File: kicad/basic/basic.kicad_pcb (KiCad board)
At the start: 2 copper layers, 50 x 50 mm, 20 parts, among them P2 CONN_01X15, P3 CONN_01X15, P4 CONN_01X06, P5 CONN_01X01, P6 CONN_01X01, P7 CONN_01X01, P8 CONN_01X01, P9 CONN_01X06, SW1 SW_PUSH, SW2 SW_PUSH

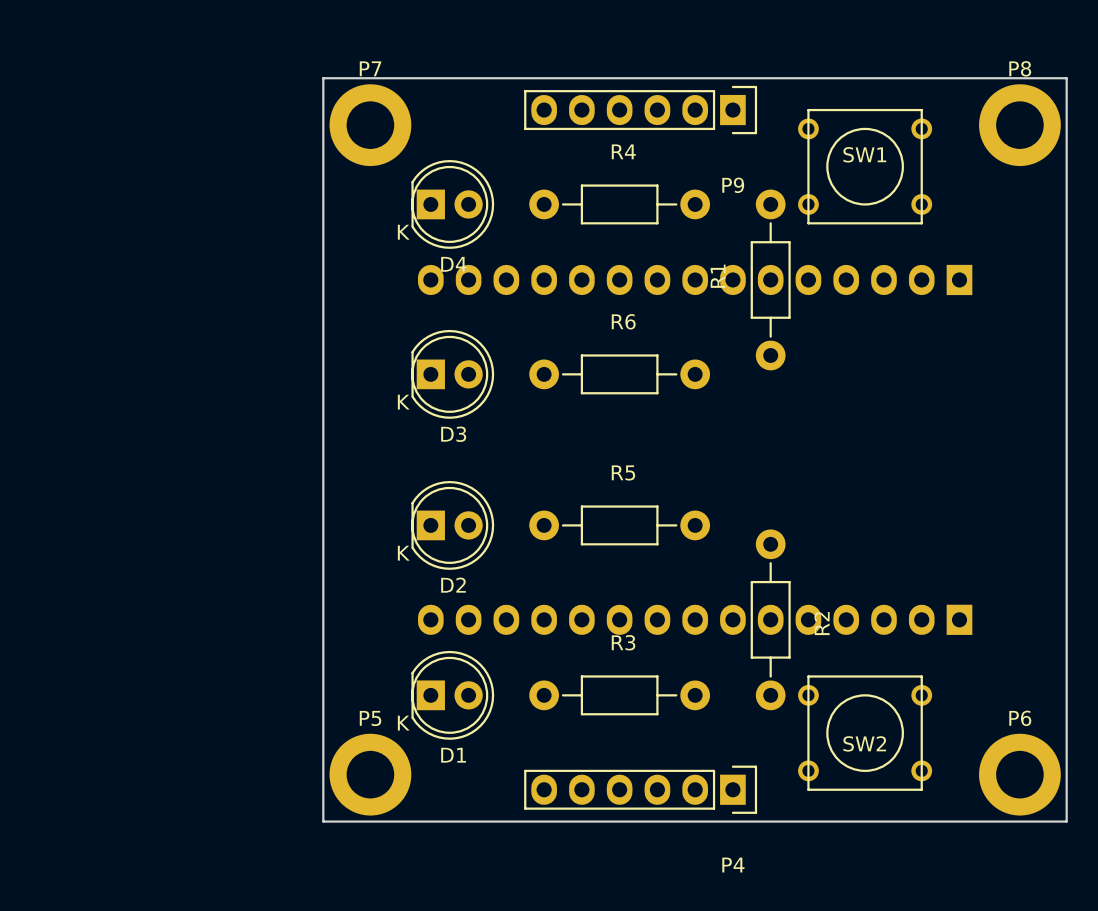
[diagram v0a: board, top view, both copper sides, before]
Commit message: Labeling
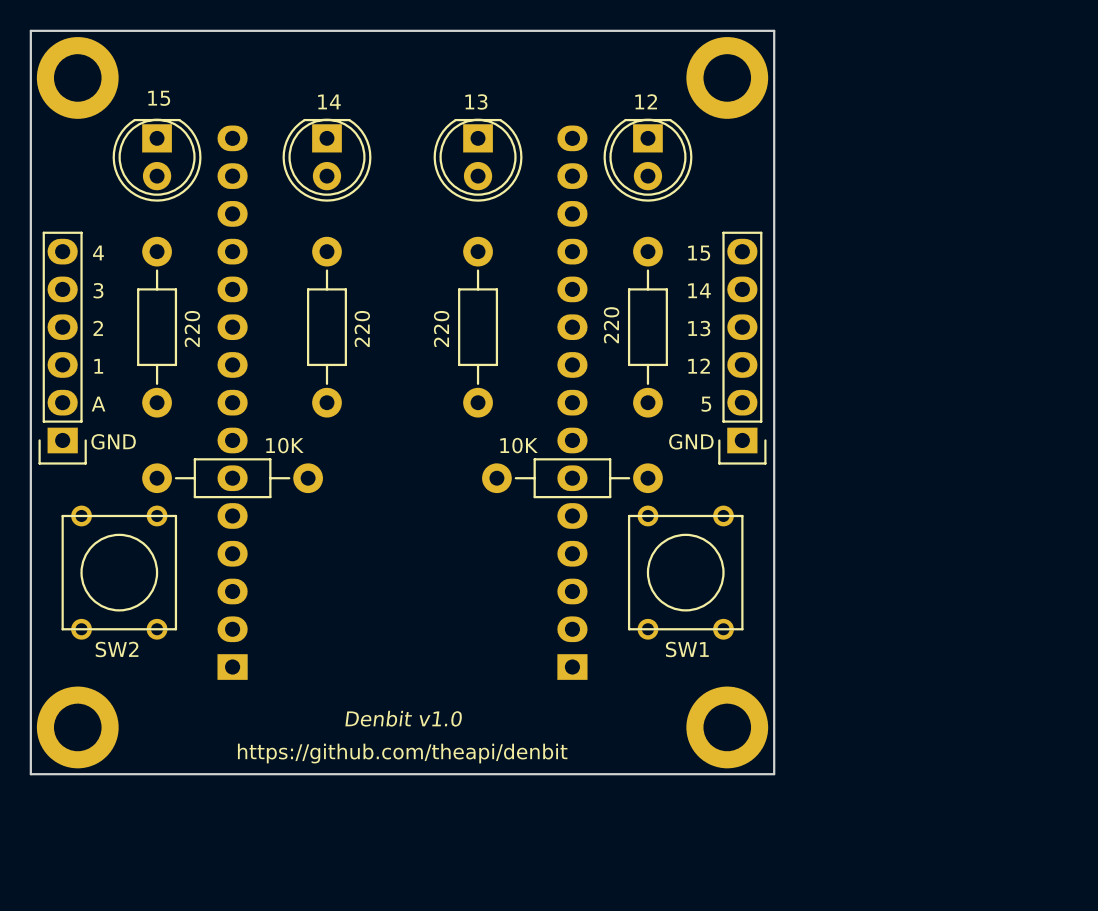
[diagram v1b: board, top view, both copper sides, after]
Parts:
- moved P6 63.5 mm to (123.5, 118.7), turned to 270 degrees
- moved SW2 51.3 mm to (126.3, 108.3), turned to 90 degrees
- moved P4 50.8 mm to (122.5, 99.4), turned to 90 degrees
- moved P5 50.8 mm to (123.5, 75.0), turned to 270 degrees
- moved P2 49.0 mm to (133.9, 114.6), turned to 90 degrees
- moved P8 45.0 mm to (167.2, 118.7), turned to 270 degrees
- moved D1 41.7 mm to (128.8, 79.0), turned to 270 degrees
- moved R3 39.6 mm to (128.8, 86.7), turned to 270 degrees
- moved P3 36.8 mm to (156.8, 114.6), turned to 90 degrees
- moved R2 31.4 mm to (139.0, 101.9), turned to 180 degrees
- moved SW1 29.9 mm to (164.4, 108.3), turned to 270 degrees
- moved D2 27.0 mm to (140.2, 79.0), turned to 270 degrees
- moved P7 24.2 mm to (167.2, 75.0), turned to 270 degrees
- moved R5 23.5 mm to (140.2, 86.7), turned to 270 degrees
- moved P9 22.2 mm to (168.2, 99.4), turned to 90 degrees
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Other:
- board text added: "1"
- board text added: "12"
- board text added: "13"
- board text added: "14"
- board text added: "15"
- board text added: "2"
- board text added: "3"
- board text added: "4"
- board text added: "5"
- board text added: "A"
- board text added: "Denbit v1.0"
- board text added: "GND"
- board text added: "https://github.com/theapi/denbit"
